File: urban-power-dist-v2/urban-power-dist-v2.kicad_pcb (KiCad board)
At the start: 2 copper layers, 27 parts, among them J1 12V_IN, J2 OUT, J3 OUT, J4 OUT, J5 TEST_PT, J6 TEST_PT, J7 TEST_PT

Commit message: layout updates
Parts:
- moved H1 129.0 mm to (75.5, 157.0)
- moved H2 120.4 mm to (75.5, 43.0)
- moved D3 100.7 mm to (156.0, 75.1), turned to 90 degrees
- moved J2 97.2 mm to (157.2, 47.5), turned to 180 degrees
- moved J4 96.2 mm to (151.8, 134.1), turned to 0 degrees
- moved D5 93.4 mm to (153.0, 106.4), turned to -90 degrees
- moved H3 93.0 mm to (236.0, 26.0)
- moved R2 91.5 mm to (156.0, 67.0), turned to 90 degrees
- moved R4 85.2 mm to (153.0, 114.5), turned to -90 degrees
- moved R5 78.0 mm to (155.0, 58.5), turned to 0 degrees
- moved R7 76.5 mm to (154.0, 123.0), turned to 180 degrees
- moved H4 68.4 mm to (236.0, 155.5)
- moved J3 67.5 mm to (212.6, 92.7), turned to 90 degrees
- moved J1 67.4 mm to (98.5, 87.3), turned to -90 degrees
- moved F3 57.3 mm to (166.2, 111.0), turned to -90 degrees
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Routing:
- net Net-(J6-Pin_1): track 17.9 -> 49.1 mm
- net Net-(J7-Pin_1): track 17.9 -> 49.1 mm
- net +12V: track 0.00 -> 30.6 mm
- net GND: track 0.00 -> 28.9 mm
- net Net-(J5-Pin_1): track 17.9 -> 35.5 mm
- net Net-(J4-Pin_1): track 23.1 -> 37.8 mm
- net Net-(J3-Pin_1): track 23.1 -> 37.8 mm
- net Net-(J2-Pin_1): track 23.1 -> 37.4 mm
- net Net-(D5-A): track 0.00 -> 5.70 mm
- net Net-(D3-A): track 0.00 -> 5.70 mm
- net Net-(D4-A): track 0.00 -> 5.70 mm
- removed copper zone on B.Cu, net GND
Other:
- board text added: "${REFERENCE}"

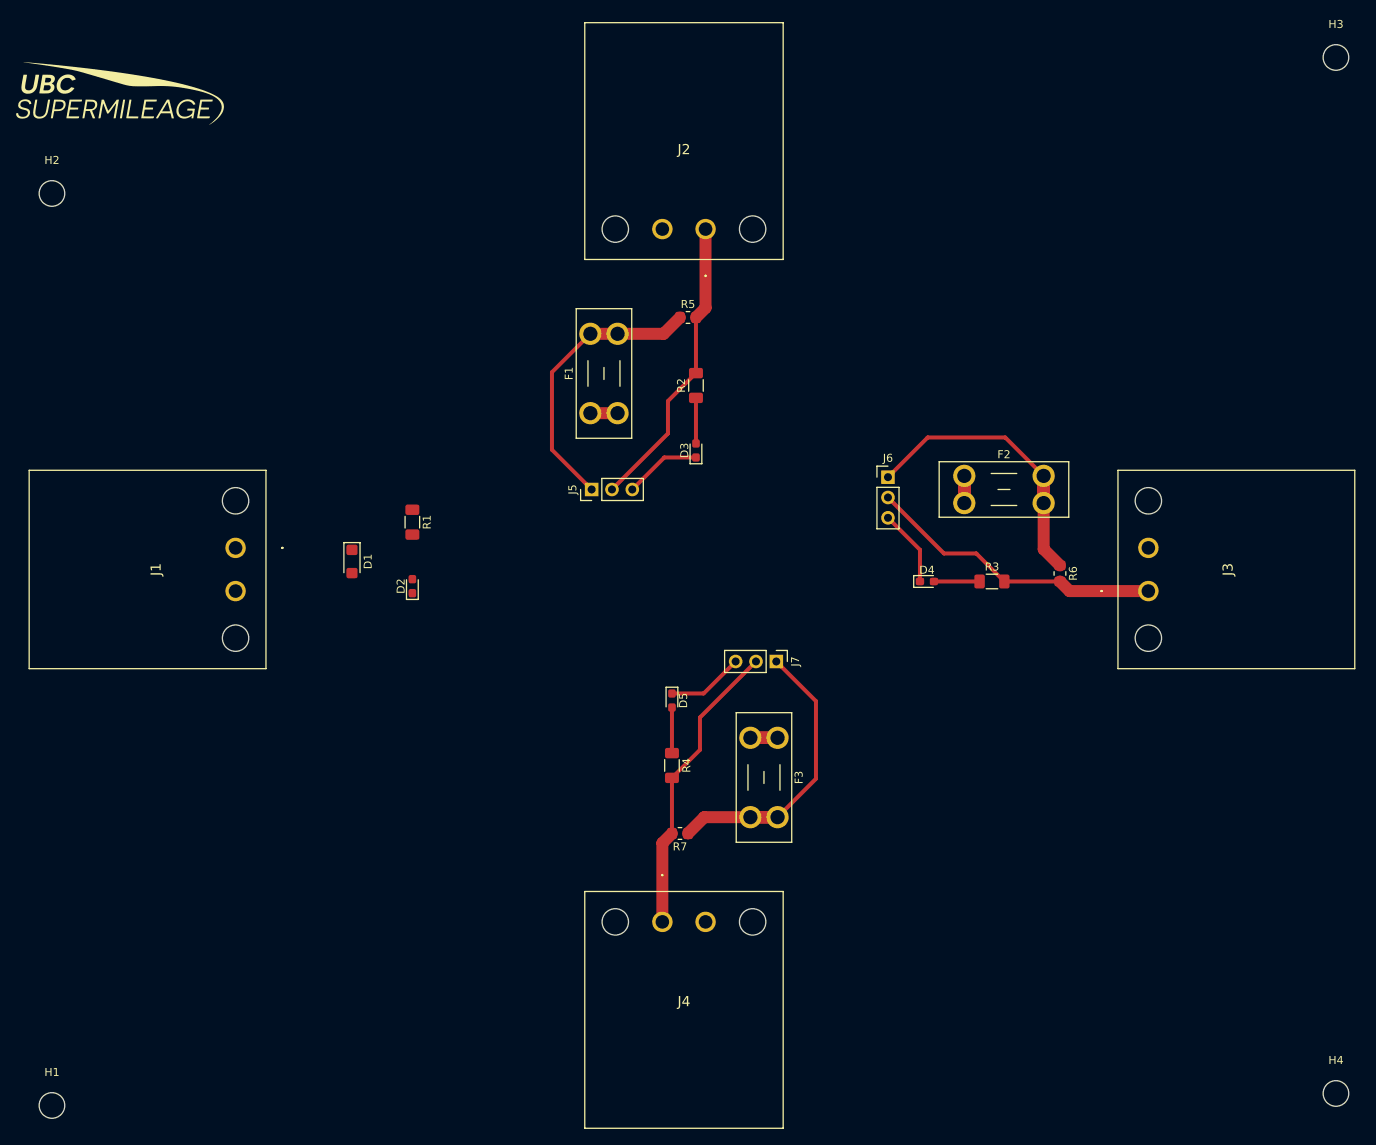
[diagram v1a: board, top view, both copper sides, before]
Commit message: close to finished layout
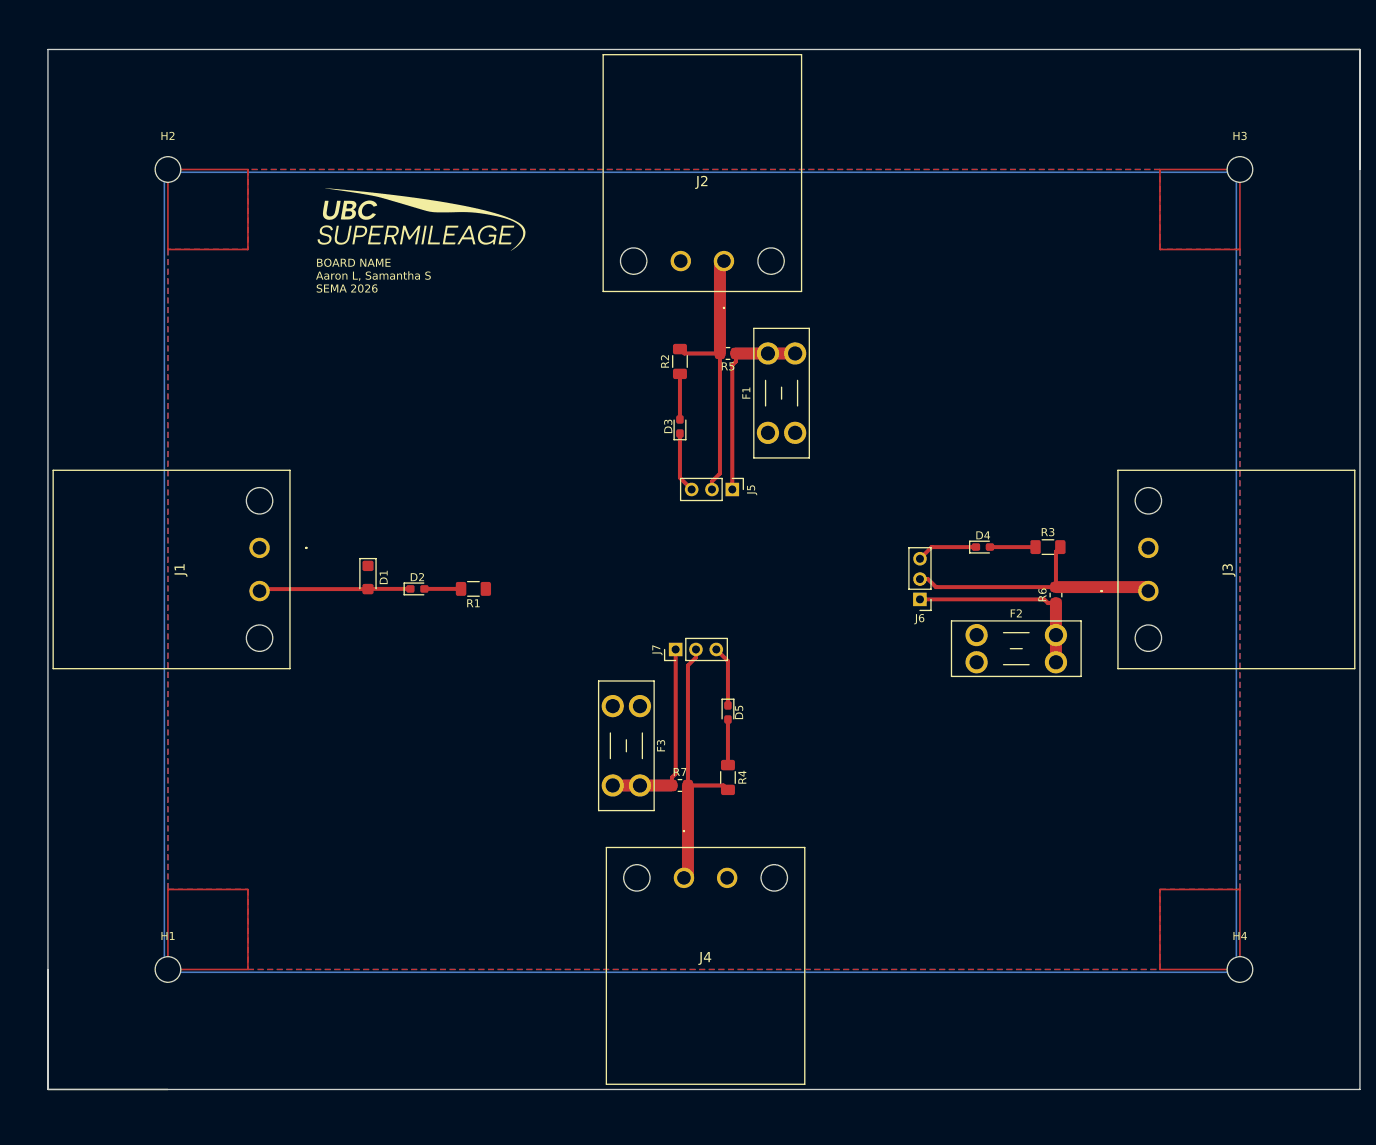
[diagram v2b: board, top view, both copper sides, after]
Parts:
- moved G*** 40.9 mm to (121.5, 47.0)
- moved H1 22.3 mm to (90.0, 140.0)
- moved F1 22.3 mm to (165.0, 72.9)
- moved F2 20.0 mm to (191.1, 98.2)
- moved H4 19.6 mm to (224.0, 140.0)
- moved H3 18.4 mm to (224.0, 40.0)
- moved F3 17.6 mm to (149.0, 107.1)
- moved J5 17.6 mm to (160.5, 80.0), turned to -90 degrees
- moved J6 15.8 mm to (184.0, 93.7), turned to 180 degrees
- moved H2 14.8 mm to (90.0, 40.0)
- moved J7 12.7 mm to (153.5, 100.0), turned to 90 degrees
- moved R1 11.3 mm to (128.2, 92.4), turned to 180 degrees
- moved D4 8.22 mm to (191.9, 87.2)
- moved R3 8.22 mm to (200.0, 87.2)
- moved D5 7.16 mm to (160.0, 107.9)
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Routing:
- net +12V: track 30.6 -> 0.00 mm
- net Net-(J6-Pin_1): track 49.1 -> 24.6 mm
- net Net-(J7-Pin_1): track 49.1 -> 24.6 mm
- net GND: track 28.9 -> 41.8 mm
- net Net-(J5-Pin_1): track 35.5 -> 24.6 mm
- net Net-(D2-A): track 0.00 -> 4.57 mm
- net Net-(J4-Pin_1): track 37.8 -> 34.8 mm
- net Net-(J3-Pin_1): track 37.8 -> 34.8 mm
- net Net-(J2-Pin_1): track 37.4 -> 34.8 mm
- added copper zone on F.Cu, net +12V
- added copper zone on B.Cu, net GND
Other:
- board outline added: 164 x 130 mm
- board text added: "BOARD NAME Aaron L, Samantha S SEMA 2026"
